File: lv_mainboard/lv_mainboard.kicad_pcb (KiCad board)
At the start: 2 copper layers, 102 x 202 mm, 21 parts, among them J1 DE9_Plug, J15 Conn_02x10_Counter_Clockwise, J16 Conn_02x10_Counter_Clockwise, J17 Conn_02x10_Counter_Clockwise, J19 Conn_02x10_Counter_Clockwise, J2 DE9_Plug, J21 Conn_02x10_Counter_Clockwise, J3 DE9_Plug, J4 DE9_Plug, J5 DE9_Plug

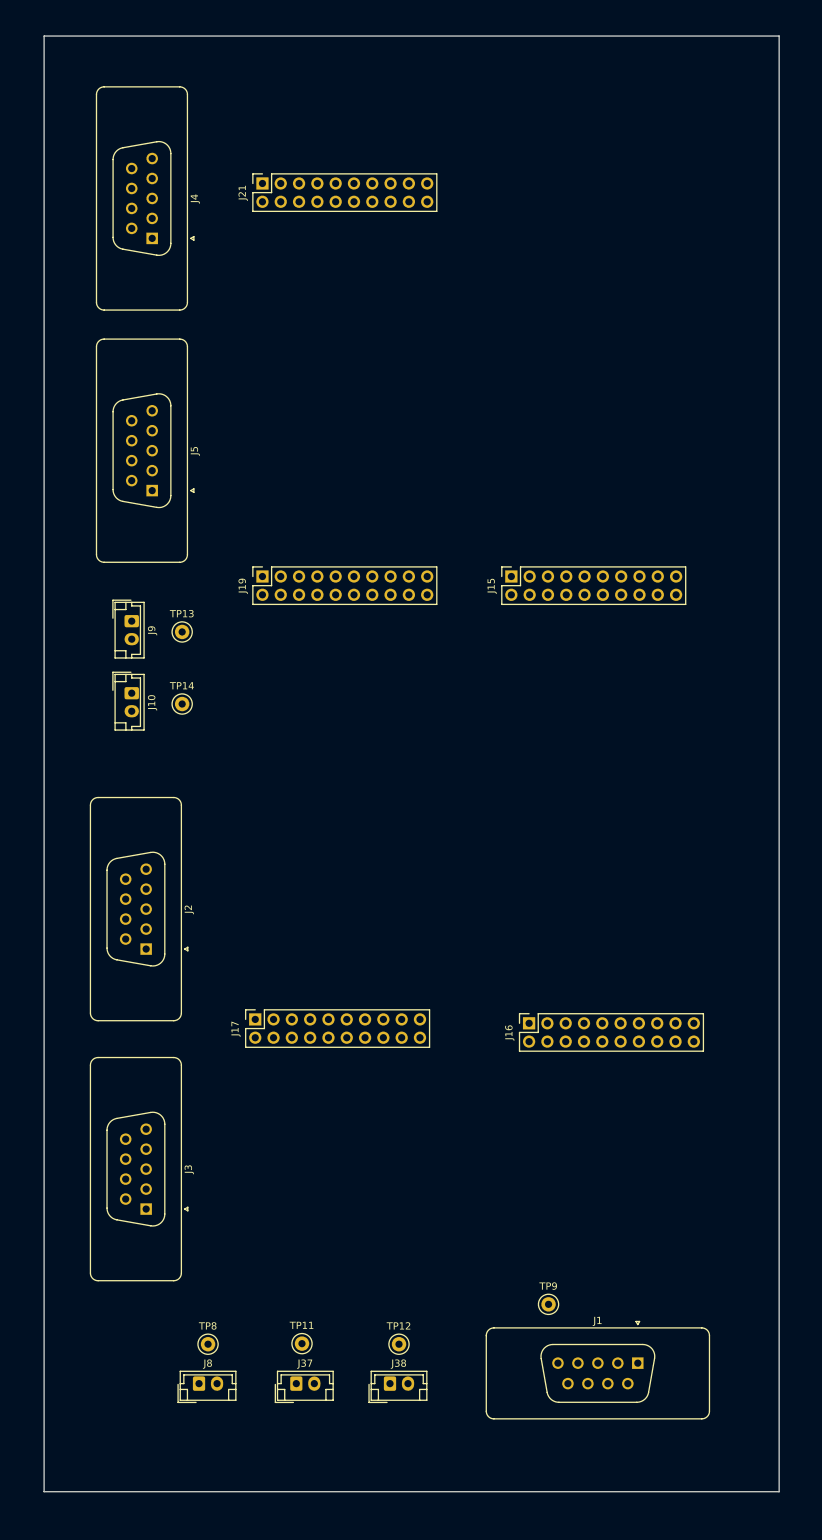
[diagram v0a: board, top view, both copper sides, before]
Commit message: add layout
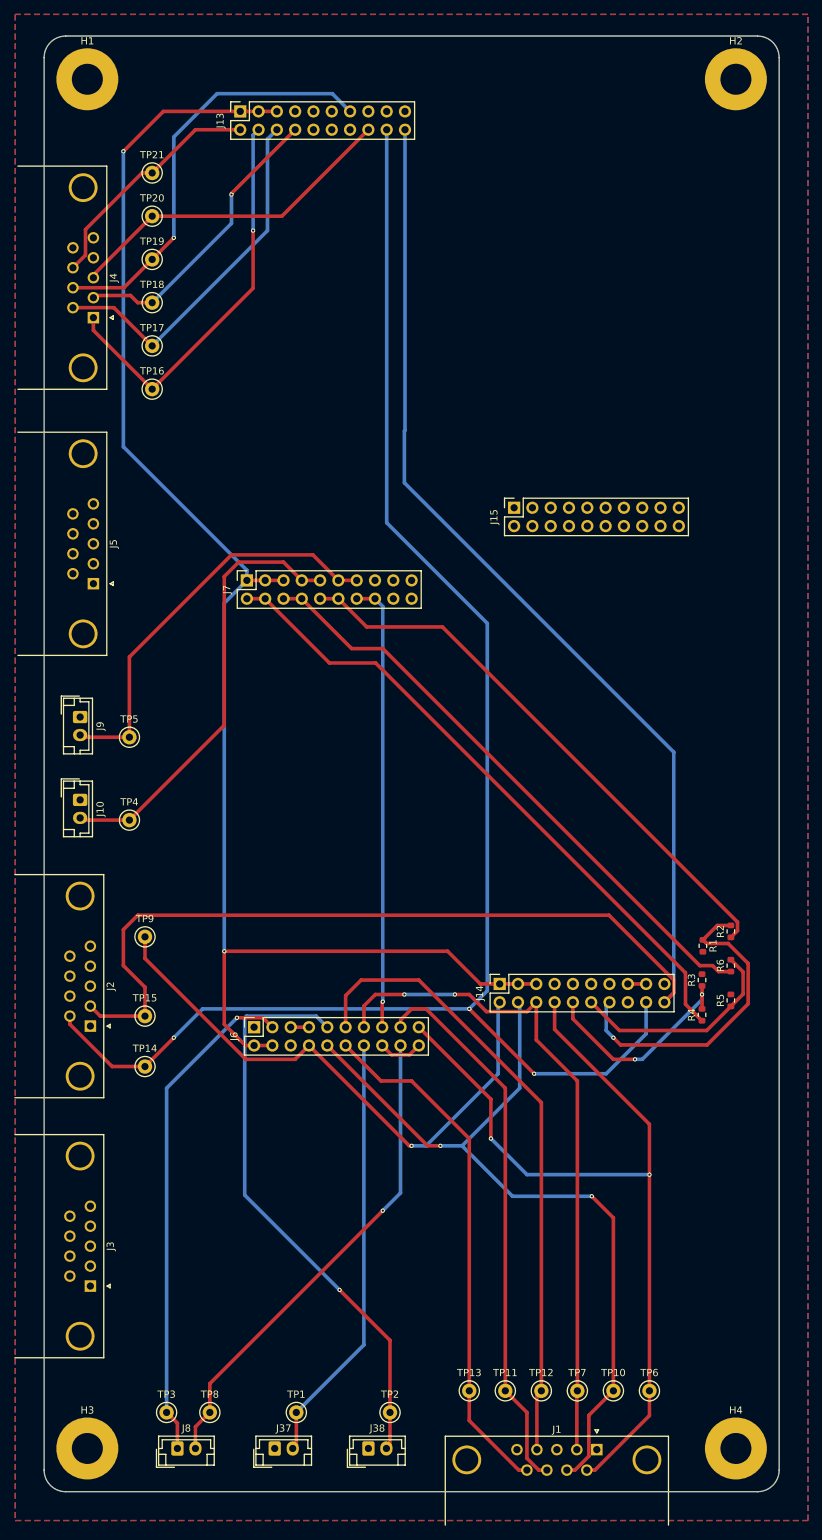
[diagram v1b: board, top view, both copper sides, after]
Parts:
- removed J16, J17, J19, J21: Conn_02x10_Counter_Clockwise, Connector_PinSocket_2.54mm:PinSocket_2x10_P2.54mm_Vertical
- added H1: MountingHole, MountingHole:MountingHole_4.3mm_M4_Pad, F.Cu at (161.0, 43.0)
- added H2: MountingHole, MountingHole:MountingHole_4.3mm_M4_Pad, F.Cu at (251.0, 43.0)
- added H3: MountingHole, MountingHole:MountingHole_4.3mm_M4_Pad, F.Cu at (161.0, 233.0)
- added H4: MountingHole, MountingHole:MountingHole_4.3mm_M4_Pad, F.Cu at (251.0, 233.0)
- added J13: Conn_02x10_Odd_Even, Connector_PinSocket_2.54mm:PinSocket_2x10_P2.54mm_Vertical, F.Cu at (182.2, 47.5)
- added J14: Conn_02x10_Odd_Even, Connector_PinSocket_2.54mm:PinSocket_2x10_P2.54mm_Vertical, F.Cu at (218.2, 168.5)
- added J6: Conn_02x10_Odd_Even, Connector_PinSocket_2.54mm:PinSocket_2x10_P2.54mm_Vertical, F.Cu at (184.1, 174.5)
- added J7: Conn_02x10_Odd_Even, Connector_PinSocket_2.54mm:PinSocket_2x10_P2.54mm_Vertical, F.Cu at (183.1, 112.5)
- added R1: 100R, Resistor_SMD:R_0603_1608Metric, F.Cu at (246.4, 163.2)
- added R2: 47R, Resistor_SMD:R_0603_1608Metric, F.Cu at (250.3, 161.2)
- added R3: 100R, Resistor_SMD:R_0603_1608Metric, F.Cu at (246.3, 168.0)
- added R4: 47R, Resistor_SMD:R_0603_1608Metric, F.Cu at (246.3, 172.8)
- added R5: 100R, Resistor_SMD:R_0603_1608Metric, F.Cu at (250.3, 170.8)
- added R6: 47R, Resistor_SMD:R_0603_1608Metric, F.Cu at (250.3, 166.0)
- added TP1: TestPoint, TestPoint:TestPoint_Keystone_5000-5004_Miniature, F.Cu at (190.0, 228.0)
- added TP10: TestPoint, TestPoint:TestPoint_Keystone_5000-5004_Miniature, F.Cu at (234.0, 225.0)
- added TP15: TestPoint, TestPoint:TestPoint_Keystone_5000-5004_Miniature, F.Cu at (169.0, 173.0)
- added TP16: TestPoint, TestPoint:TestPoint_Keystone_5000-5004_Miniature, F.Cu at (170.0, 86.0)
- added TP17: TestPoint, TestPoint:TestPoint_Keystone_5000-5004_Miniature, F.Cu at (170.0, 80.0)
- added TP18: TestPoint, TestPoint:TestPoint_Keystone_5000-5004_Miniature, F.Cu at (170.0, 74.0)
- added TP19: TestPoint, TestPoint:TestPoint_Keystone_5000-5004_Miniature, F.Cu at (170.0, 68.0)
- added TP2: TestPoint, TestPoint:TestPoint_Keystone_5000-5004_Miniature, F.Cu at (203.0, 228.0)
- added TP20: TestPoint, TestPoint:TestPoint_Keystone_5000-5004_Miniature, F.Cu at (170.0, 62.0)
- added TP21: TestPoint, TestPoint:TestPoint_Keystone_5000-5004_Miniature, F.Cu at (170.0, 56.0)
- added TP3: TestPoint, TestPoint:TestPoint_Keystone_5000-5004_Miniature, F.Cu at (172.0, 228.0)
- added TP4: TestPoint, TestPoint:TestPoint_Keystone_5000-5004_Miniature, F.Cu at (166.8, 145.8)
- added TP5: TestPoint, TestPoint:TestPoint_Keystone_5000-5004_Miniature, F.Cu at (166.8, 134.3)
- added TP6: TestPoint, TestPoint:TestPoint_Keystone_5000-5004_Miniature, F.Cu at (239.0, 225.0)
- added TP7: TestPoint, TestPoint:TestPoint_Keystone_5000-5004_Miniature, F.Cu at (229.0, 225.0)
- J1, J2, J3, J4, J5: footprint Connector_Dsub:DSUB-9_Female_Vertical_P2.77x2.84mm -> Connector_Dsub:DSUB-9_Female_Horizontal_P2.77x2.84mm_EdgePinOffset7.70mm_Housed_MountingHolesOffset9.12mm
- moved TP13 112.6 mm to (214.0, 225.0)
- moved TP9 75.7 mm to (169.0, 162.0)
- moved TP14 50.6 mm to (169.0, 180.0)
- moved TP11 29.0 mm to (219.0, 225.0)
- moved TP12 20.8 mm to (224.0, 225.0)
- moved J10 16.4 mm to (160.0, 143.0)
- moved J5 15.3 mm to (161.8, 113.0)
- moved J9 15.1 mm to (160.0, 131.5)
- moved J4 13.7 mm to (161.8, 76.1)
- moved J1 13.3 mm to (231.7, 233.2)
- moved J2 13.2 mm to (161.4, 174.4)
- moved J3 13.2 mm to (161.4, 210.5)
- moved J15 9.55 mm to (220.2, 102.5)
- moved J37 9.49 mm to (187.0, 233.0)
- moved J38 9.49 mm to (200.0, 233.0)
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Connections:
- net Net-(J8-Pin_2) renamed BSPD_IN
- J1 pad 1: unconnected-(J1-Pad1) -> +12V
- J1 pad 2: unconnected-(J1-Pad2) -> IMD_LED
- J1 pad 4: unconnected-(J1-Pad4) -> IMD_RST
- J1 pad 5: unconnected-(J1-Pad5) -> GND
- J1 pad 6: unconnected-(J1-Pad6) -> BSPD_LED
- J1 pad 7: unconnected-(J1-Pad7) -> BMS_LED
- J1 pad 8: unconnected-(J1-Pad8) -> BSPD_RST
- J1 pad 9: unconnected-(J1-Pad9) -> BMS_RST
- J10 pad 2: Net-(J10-Pin_2) -> Brake_init
- J2 pad 1: unconnected-(J2-Pad1) -> +24V
- J2 pad 2: unconnected-(J2-Pad2) -> CAN+
- J2 pad 5: unconnected-(J2-Pad5) -> GND
- J2 pad 6: unconnected-(J2-Pad6) -> CAN-
- J37 pad 2: Net-(J37-Pin_2) -> IMD_FAULT
- J38 pad 2: Net-(J38-Pin_2) -> BMS_FAULT
- J4 pad 1: unconnected-(J4-Pad1) -> FAN_PWM
- J4 pad 2: unconnected-(J4-Pad2) -> PT_signal
- J4 pad 3: unconnected-(J4-Pad3) -> USART1
- J4 pad 5: unconnected-(J4-Pad5) -> GND
- J4 pad 6: unconnected-(J4-Pad6) -> PUMP_PWM
- J4 pad 7: unconnected-(J4-Pad7) -> TIM1_CH1
- J4 pad 8: unconnected-(J4-Pad8) -> USART2
- J8 pad 1: GND -> SW_OUT
- J9 pad 2: Net-(J9-Pin_2) -> Current_init
- TP11 pad 1: Net-(J37-Pin_2) -> BSPD_RST
- TP12 pad 1: Net-(J38-Pin_2) -> IMD_RST
- TP13 pad 1: Net-(J9-Pin_2) -> BMS_RST
- TP14 pad 1: Net-(J10-Pin_2) -> CAN-
- TP9 pad 1: unconnected-(TP9-Pad1) -> SW_Fault
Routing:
- net CAN+: track 0.00 -> 243.1 mm
- net CAN-: track 0.00 -> 226.1 mm, vias 0 -> 3
- net VDC: track 0.00 -> 211.3 mm, vias 0 -> 2
- net BSPD_LED: track 0.00 -> 118.3 mm, vias 0 -> 2
- net BMS_LED: track 0.00 -> 111.3 mm, vias 0 -> 2
- net IMD_LED: track 0.00 -> 93.5 mm, vias 0 -> 2
- net Brake_Limit_Check_out: track 0.00 -> 90.0 mm
- net IMD_RST: track 0.00 -> 87.9 mm
- net Current_Limit_Check_out: track 0.00 -> 83.5 mm
- net BMS_FAULT: track 0.00 -> 80.5 mm, vias 0 -> 1
- net Simultaneous_brake&current: track 0.00 -> 78.8 mm
- net SW_Fault: track 0.00 -> 78.5 mm, vias 0 -> 1
- net BSPD_RST: track 0.00 -> 76.8 mm
- net BMS_RST: track 0.00 -> 72.5 mm
- net SW_OUT: track 0.00 -> 69.9 mm, vias 0 -> 1
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- added copper zone on B.Cu, net GND
- added copper zone on F.Cu, net GND
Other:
- outline, holes or cut-outs redrawn
